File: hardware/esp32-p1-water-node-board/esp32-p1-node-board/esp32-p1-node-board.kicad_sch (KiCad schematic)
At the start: 15 parts, among them J1 RJ11-6, J2 Conn_01x03, Q1 BSS138, Q3 BC847

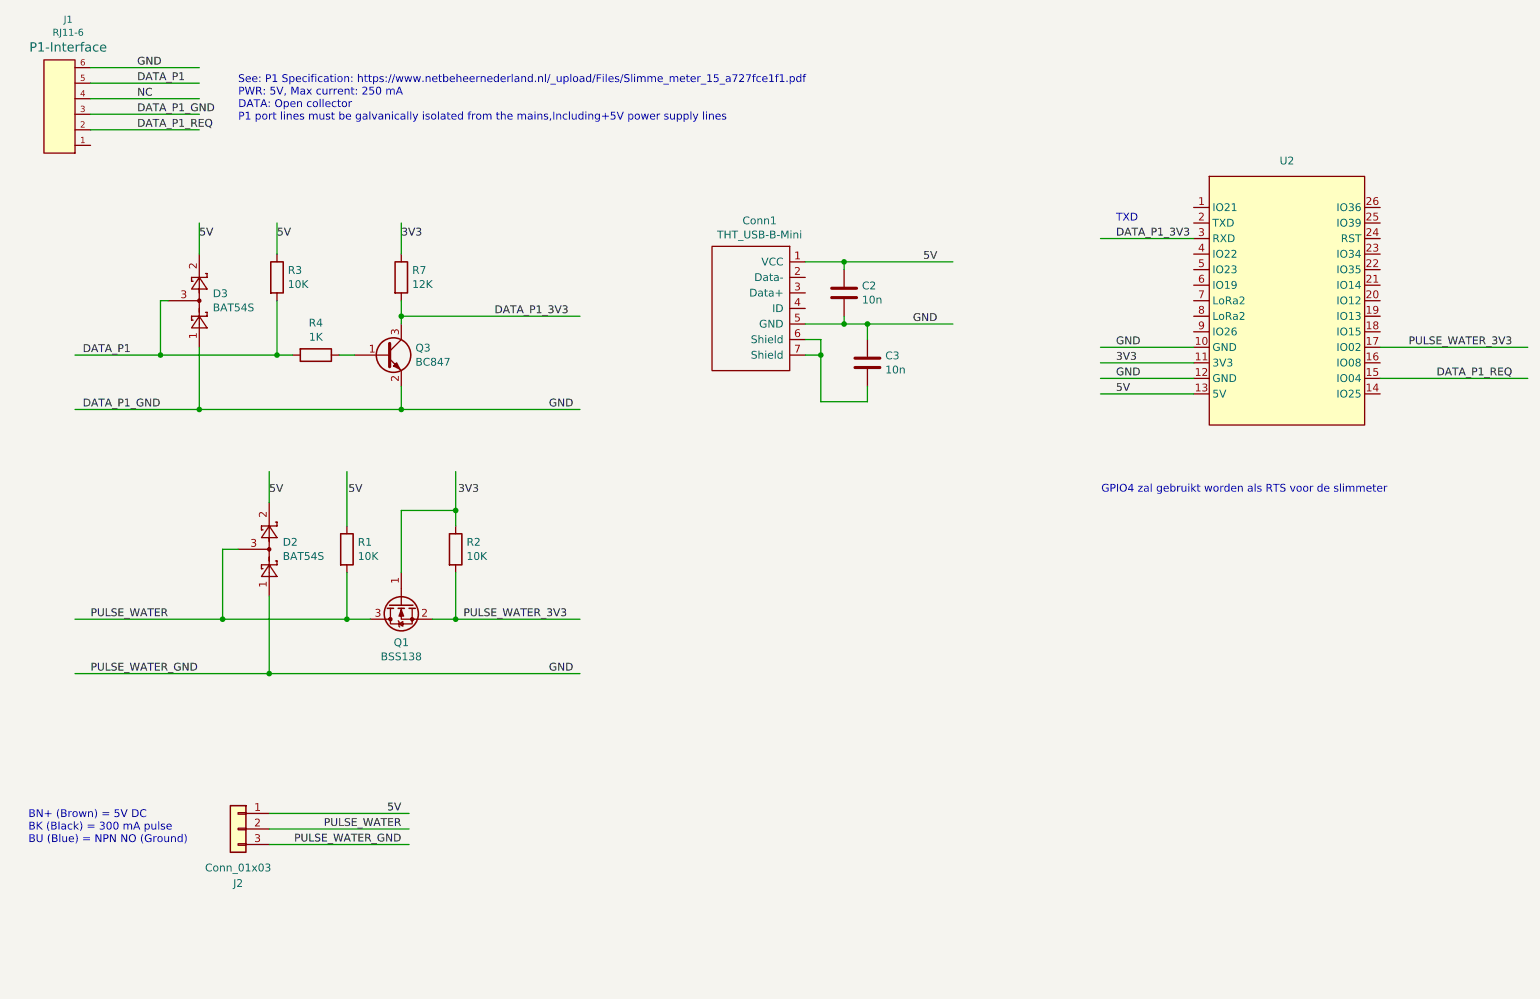
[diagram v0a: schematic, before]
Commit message: Start design PCB
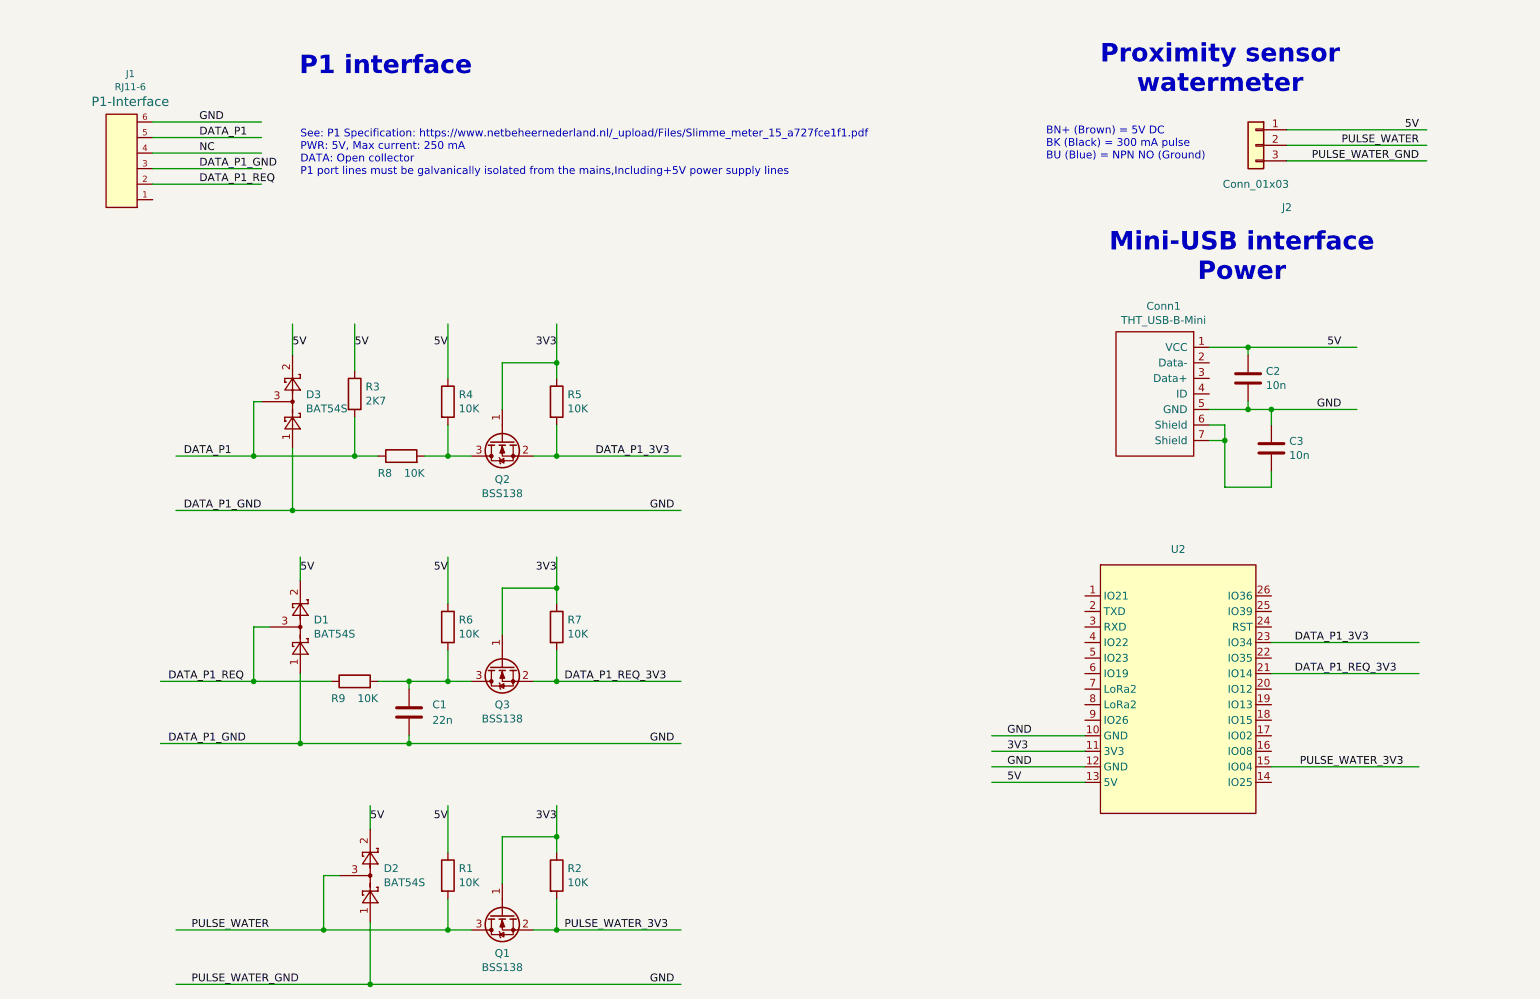
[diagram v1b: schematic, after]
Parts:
- removed Q3: BC847, Package_TO_SOT_SMD:SOT-23, symbol Transistor_BJT:BC847
- added C1: 22n, Capacitor_SMD:C_1206_3216Metric, symbol Device:C
- added D1: BAT54S, Package_TO_SOT_SMD:SOT-23, symbol esp32-p1-node-board-rescue:BAT54S-Diode
- added Q2, Q3: BSS138, Package_TO_SOT_SMD:SOT-23, symbol Transistor_FET:BSS138
- added R5, R6, R8, R9: 10K, Resistor_SMD:R_1206_3216Metric, symbol Device:R
- R3: value 10K -> 2K7
- R4: value 1K -> 10K
- R7: value 12K -> 10K
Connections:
- net 3V3: now also Q1.1 (G), R2.1, Q2.1 (G), Q3.1 (G), R5.1
- net 5V: now also R1.1, R4.1, D1.2, R6.1
- net DATA_P1: now also R8.1; no longer R4.2
- net DATA_P1_3V3: now also U2.23 (IO34), Q2.2 (S), R5.2; no longer R7.2, U2.3 (RXD)
- net DATA_P1_GND: now also C1.2, D1.1
- net DATA_P1_REQ: now also D1.3, R9.1; no longer U2.15 (IO04)
- net PULSE_WATER_3V3: now also U2.15 (IO04); no longer U2.17 (IO02)
- net DATA_P1_REQ_3V3: now reaches U2.21 (IO14)
- net DATA_P1_REQ_3V3: now also R7.2, Q3.2 (S)
- new net: C1.1, Q3.3 (D), R6.2, R9.2
- new net: Q2.3 (D), R4.2, R8.2
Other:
- note added: "Mini-USB interface Power"
- note added: "P1 interface"
- note added: "Proximity sensor watermeter"
- note removed: "GPIO4 zal gebruikt worden als RTS voor de slimmeter"
- note removed: "TXD"
- moved on the sheet: C2, C3, Conn1, D2, D3, J1, J2, Q1, R1, R2, R3, U2
